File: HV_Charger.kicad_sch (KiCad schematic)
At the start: 25 parts, among them J1 HVIL, J10 G6B-1114P-US-DC24, J11 Banana_Connector, J12 Battery GLV, J2 E-Stop, J3 PP Connector, J4 IMD Indicator, J5 AMS Indicator, J6 CAN, J7 CAN_Expansion1, J8 CAN_Expansion2, J9 DC Input

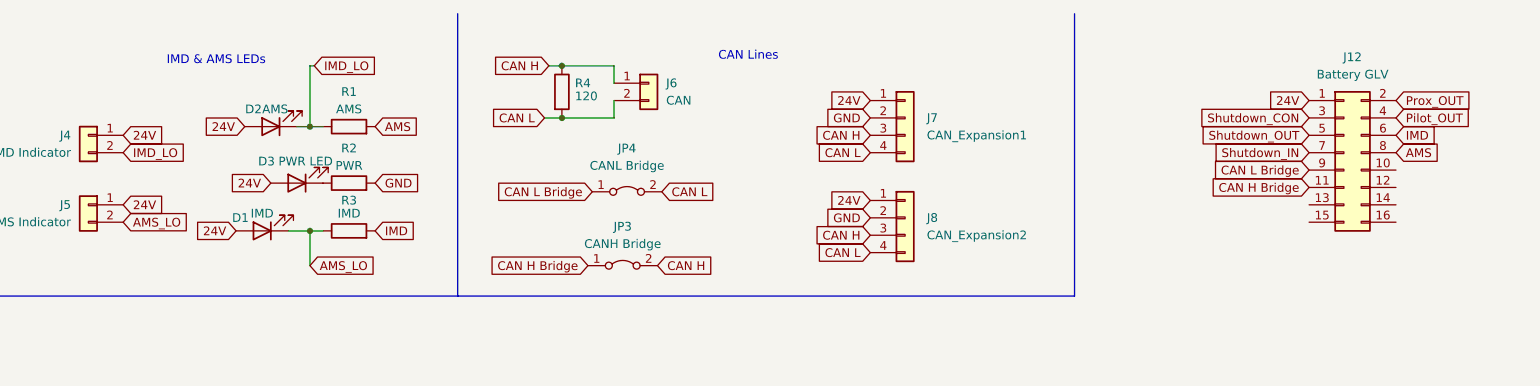
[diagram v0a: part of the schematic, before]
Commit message: more stuff done
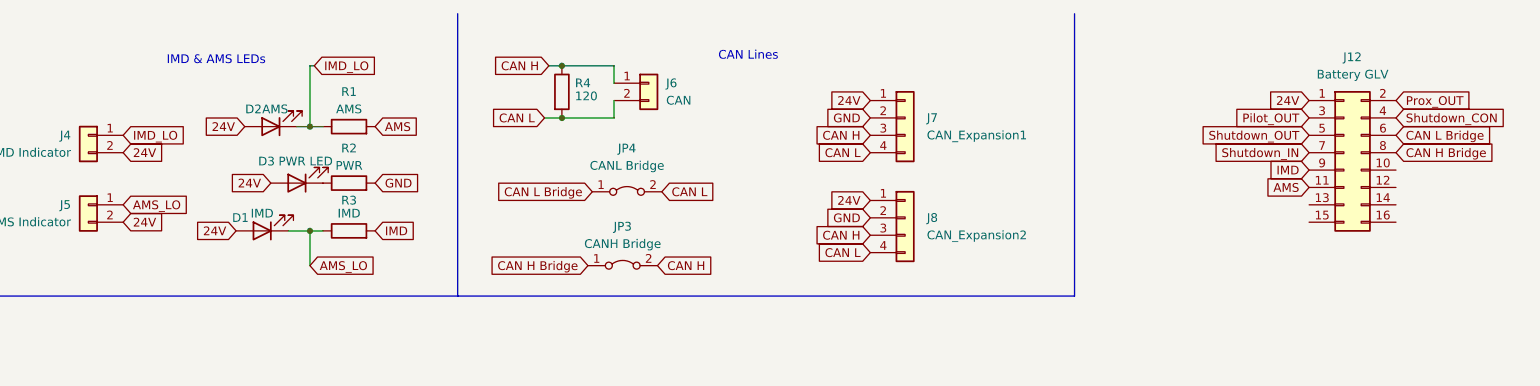
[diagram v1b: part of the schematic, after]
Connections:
- net 24V: now also J4.2 (Pin_2), J5.2 (Pin_2); no longer J4.1 (Pin_1), J5.1 (Pin_1)
- net AMS: now also J12.11 (Pin_11); no longer J12.8 (Pin_8)
- net AMS_LO: now also J5.1 (Pin_1); no longer J5.2 (Pin_2)
- net CAN H Bridge: now also J12.8 (Pin_8); no longer J12.11 (Pin_11)
- net CAN L Bridge: now also J12.6 (Pin_6); no longer J12.9 (Pin_9)
- net IMD: now also J12.9 (Pin_9); no longer J12.6 (Pin_6)
- net IMD_LO: now also J4.1 (Pin_1); no longer J4.2 (Pin_2)
- net Pilot_OUT: now also J12.3 (Pin_3); no longer J12.4 (Pin_4)
- net Shutdown_CON: now also J12.4 (Pin_4); no longer J12.3 (Pin_3)
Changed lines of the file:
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@@
     (effects (font (size 1.27 1.27)) (justify left bottom))
   )
-  (global_label "Pilot_OUT" (shape input) (at 269.24 27.305 0) (fields_autoplaced)
-    (effects (font (size 1.27 1.27)) (justify left))
-    (property "Intersheet References" "${INTERSHEET_REFS}" (id 0) (at 280.6641 27.2256 0)
-      (effects (font (size 1.27 1.27)) (justify left) hide)
-    )
-  )
   (global_label "Shutdown_IN" (shape input) (at 256.54 32.385 180) (fields_autoplaced)
     (effects (font (size 1.27 1.27)) (justify right))
@@
     )
   )
-  (global_label "AMS_LO" (shape input) (at 83.185 42.545 0) (fields_autoplaced)
-    (effects (font (size 1.27 1.27)) (justify left))
-    (property "Intersheet References" "${INTERSHEET_REFS}" (id 0) (at 92.6738 42.4656 0)
-      (effects (font (size 1.27 1.27)) (justify left) hide)
-    )
-  )
   (global_label "GND" (shape input) (at 192.405 41.91 180) (fields_autoplaced)
     (effects (font (size 1.27 1.27)) (justify right))
@@
     )
   )
-  (global_label "CAN H Bridge" (shape input) (at 256.54 37.465 180) (fields_autoplaced)
-    (effects (font (size 1.27 1.27)) (justify right))
-    (property "Intersheet References" "${INTERSHEET_REFS}" (id 0) (at 241.1245 37.3856 0)
-      (effects (font (size 1.27 1.27)) (justify right) hide)
+  (global_label "24V" (shape input) (at 83.185 32.385 0) (fields_autoplaced)
+    (effects (font (size 1.27 1.27)) (justify left))
+    (property "Intersheet References" "${INTERSHEET_REFS}" (id 0) (at 89.1057 32.3056 0)
+      (effects (font (size 1.27 1.27)) (justify left) hide)
     )
   )
@@
     )
   )
+  (global_label "IMD_LO" (shape input) (at 83.185 29.845 0) (fields_autoplaced)
+    (effects (font (size 1.27 1.27)) (justify left))
+    (property "Intersheet References" "${INTERSHEET_REFS}" (id 0) (at 92.2505 29.7656 0)
+      (effects (font (size 1.27 1.27)) (justify left) hide)
+    )
+  )
   (global_label "24V" (shape input) (at 256.54 24.765 180) (fields_autoplaced)
     (effects (font (size 1.27 1.27)) (justify right))
@@
     )
   )
-  (global_label "24V" (shape input) (at 83.185 40.005 0) (fields_autoplaced)
-    (effects (font (size 1.27 1.27)) (justify left))
-    (property "Intersheet References" "${INTERSHEET_REFS}" (id 0) (at 89.1057 39.9256 0)
-      (effects (font (size 1.27 1.27)) (justify left) hide)
-    )
-  )
   (global_label "CAN H" (shape input) (at 192.405 29.845 180) (fields_autoplaced)
     (effects (font (size 1.27 1.27)) (justify right))
@@
     )
   )
+  (global_label "AMS" (shape input) (at 256.54 37.465 180) (fields_autoplaced)
+    (effects (font (size 1.27 1.27)) (justify right))
+    (property "Intersheet References" "${INTERSHEET_REFS}" (id 0) (at 250.3774 37.5444 0)
+      (effects (font (size 1.27 1.27)) (justify right) hide)
+    )
+  )
   (global_label "24V" (shape input) (at 192.405 24.765 180) (fields_autoplaced)
     (effects (font (size 1.27 1.27)) (justify right))
@@
     )
   )
+  (global_label "CAN L Bridge" (shape input) (at 269.24 29.845 0) (fields_autoplaced)
+    (effects (font (size 1.27 1.27)) (justify left))
+    (property "Intersheet References" "${INTERSHEET_REFS}" (id 0) (at 284.3531 29.9244 0)
+      (effects (font (size 1.27 1.27)) (justify left) hide)
+    )
+  )
   (global_label "CAN L Bridge" (shape input) (at 151.765 38.1 180) (fields_autoplaced)
     (effects (font (size 1.27 1.27)) (justify right))
@@
     )
   )
-  (global_label "24V" (shape input) (at 83.185 29.845 0) (fields_autoplaced)
-    (effects (font (size 1.27 1.27)) (justify left))
-    (property "Intersheet References" "${INTERSHEET_REFS}" (id 0) (at 89.1057 29.7656 0)
-      (effects (font (size 1.27 1.27)) (justify left) hide)
-    )
-  )
   (global_label "24V" (shape input) (at 100.965 28.575 180) (fields_autoplaced)
     (effects (font (size 1.27 1.27)) (justify right))
@@
     )
   )
+  (global_label "Shutdown_CON" (shape input) (at 269.24 27.305 0) (fields_autoplaced)
+    (effects (font (size 1.27 1.27)) (justify left))
+    (property "Intersheet References" "${INTERSHEET_REFS}" (id 0) (at 285.5626 27.3844 0)
+      (effects (font (size 1.27 1.27)) (justify left) hide)
+    )
+  )
   (global_label "CAN L" (shape input) (at 192.405 32.385 180) (fields_autoplaced)
     (effects (font (size 1.27 1.27)) (justify right))
@@
     )
   )
+  (global_label "24V" (shape input) (at 83.185 42.545 0) (fields_autoplaced)
+    (effects (font (size 1.27 1.27)) (justify left))
+    (property "Intersheet References" "${INTERSHEET_REFS}" (id 0) (at 89.1057 42.4656 0)
+      (effects (font (size 1.27 1.27)) (justify left) hide)
+    )
+  )
   (global_label "Prox" (shape input) (at 27.94 66.675 180) (fields_autoplaced)
     (effects (font (size 1.27 1.27)) (justify right))
@@
     )
   )
+  (global_label "AMS_LO" (shape input) (at 83.185 40.005 0) (fields_autoplaced)
+    (effects (font (size 1.27 1.27)) (justify left))
+    (property "Intersheet References" "${INTERSHEET_REFS}" (id 0) (at 92.6738 39.9256 0)
+      (effects (font (size 1.27 1.27)) (justify left) hide)
+    )
+  )
   (global_label "Shutdown_OUT" (shape input) (at 256.54 29.845 180) (fields_autoplaced)
     (effects (font (size 1.27 1.27)) (justify right))
@@
     )
   )
+  (global_label "IMD" (shape input) (at 256.54 34.925 180) (fields_autoplaced)
+    (effects (font (size 1.27 1.27)) (justify right))
+    (property "Intersheet References" "${INTERSHEET_REFS}" (id 0) (at 250.8007 35.0044 0)
+      (effects (font (size 1.27 1.27)) (justify right) hide)
+    )
+  )
   (global_label "Prox_OUT" (shape input) (at 269.24 24.765 0) (fields_autoplaced)
     (effects (font (size 1.27 1.27)) (justify left))
@@
     )
   )
-  (global_label "IMD" (shape input) (at 269.24 29.845 0) (fields_autoplaced)
-    (effects (font (size 1.27 1.27)) (justify left))
-    (property "Intersheet References" "${INTERSHEET_REFS}" (id 0) (at 274.9793 29.7656 0)
-      (effects (font (size 1.27 1.27)) (justify left) hide)
-    )
-  )
-  (global_label "Shutdown_CON" (shape input) (at 256.54 27.305 180) (fields_autoplaced)
-    (effects (font (size 1.27 1.27)) (justify right))
-    (property "Intersheet References" "${INTERSHEET_REFS}" (id 0) (at 240.2174 27.2256 0)
+  (global_label "Pilot_OUT" (shape input) (at 256.54 27.305 180) (fields_autoplaced)
+    (effects (font (size 1.27 1.27)) (justify right))
+    (property "Intersheet References" "${INTERSHEET_REFS}" (id 0) (at 245.1159 27.3844 0)
       (effects (font (size 1.27 1.27)) (justify right) hide)
     )
@@
     )
   )
-  (global_label "CAN L Bridge" (shape input) (at 256.54 34.925 180) (fields_autoplaced)
-    (effects (font (size 1.27 1.27)) (justify right))
-    (property "Intersheet References" "${INTERSHEET_REFS}" (id 0) (at 241.4269 34.8456 0)
-      (effects (font (size 1.27 1.27)) (justify right) hide)
-    )
-  )
   (global_label "24V" (shape input) (at 33.655 24.765 0) (fields_autoplaced)
     (effects (font (size 1.27 1.27)) (justify left))
@@
     )
   )
-  (global_label "IMD_LO" (shape input) (at 83.185 32.385 0) (fields_autoplaced)
-    (effects (font (size 1.27 1.27)) (justify left))
-    (property "Intersheet References" "${INTERSHEET_REFS}" (id 0) (at 92.2505 32.3056 0)
-      (effects (font (size 1.27 1.27)) (justify left) hide)
-    )
-  )
   (global_label "Pilot" (shape input) (at 220.345 152.4 180) (fields_autoplaced)
     (effects (font (size 1.27 1.27)) (justify right))
@@
     )
   )
-  (global_label "AMS" (shape input) (at 269.24 32.385 0) (fields_autoplaced)
-    (effects (font (size 1.27 1.27)) (justify left))
-    (property "Intersheet References" "${INTERSHEET_REFS}" (id 0) (at 275.4026 32.3056 0)
-      (effects (font (size 1.27 1.27)) (justify left) hide)
-    )
+  (global_label "CAN H Bridge" (shape input) (at 269.24 32.385 0) (fields_autoplaced)
+    (effects (font (size 1.27 1.27)) (justify left))
+    (property "Intersheet References" "${INTERSHEET_REFS}" (id 0) (at 284.6555 32.4644 0)
+      (effects (font (size 1.27 1.27)) (justify left) hide)
+    )

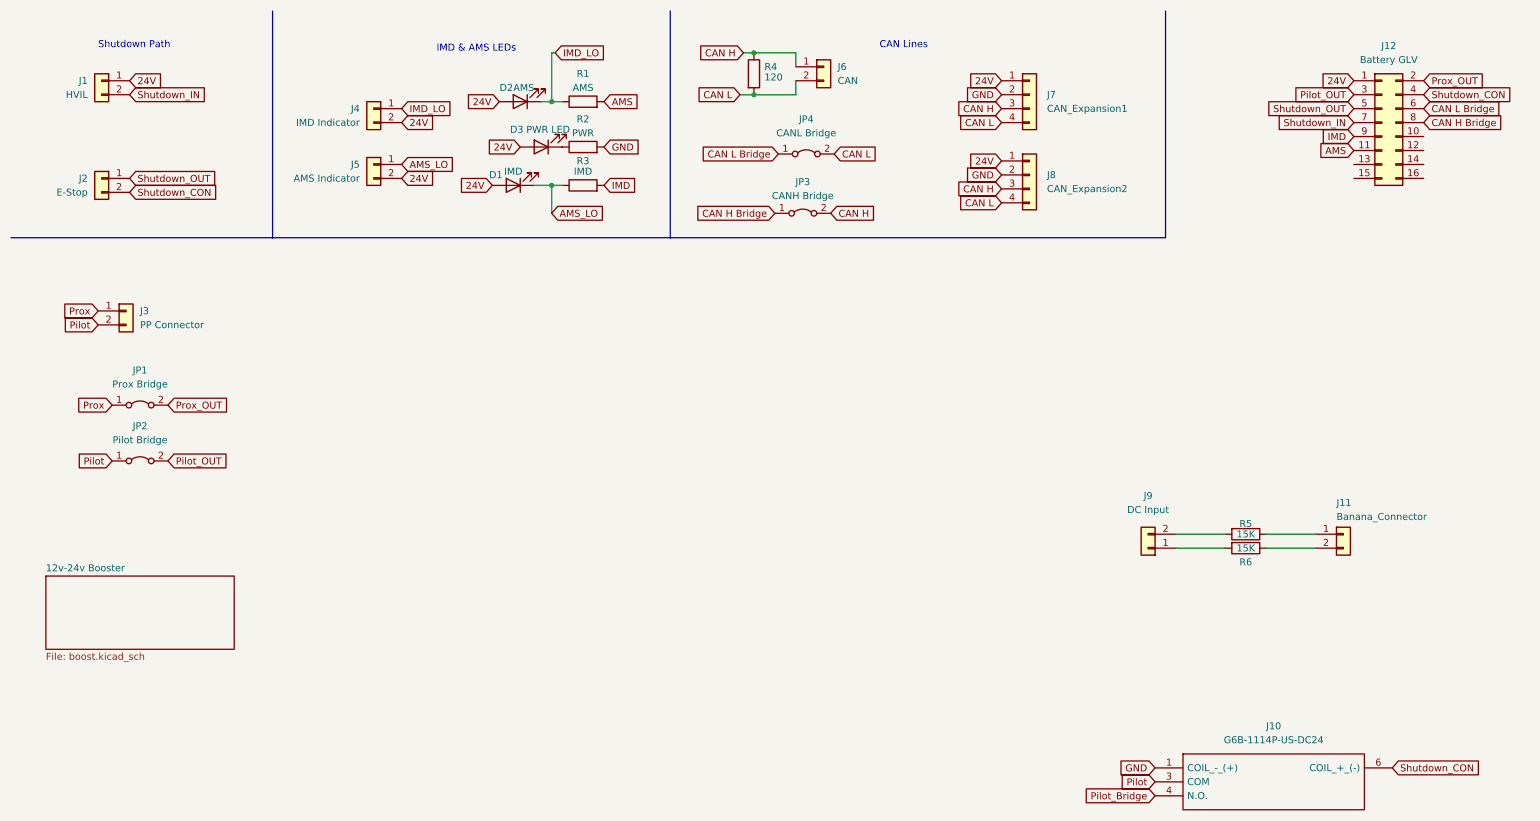
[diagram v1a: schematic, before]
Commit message: Done
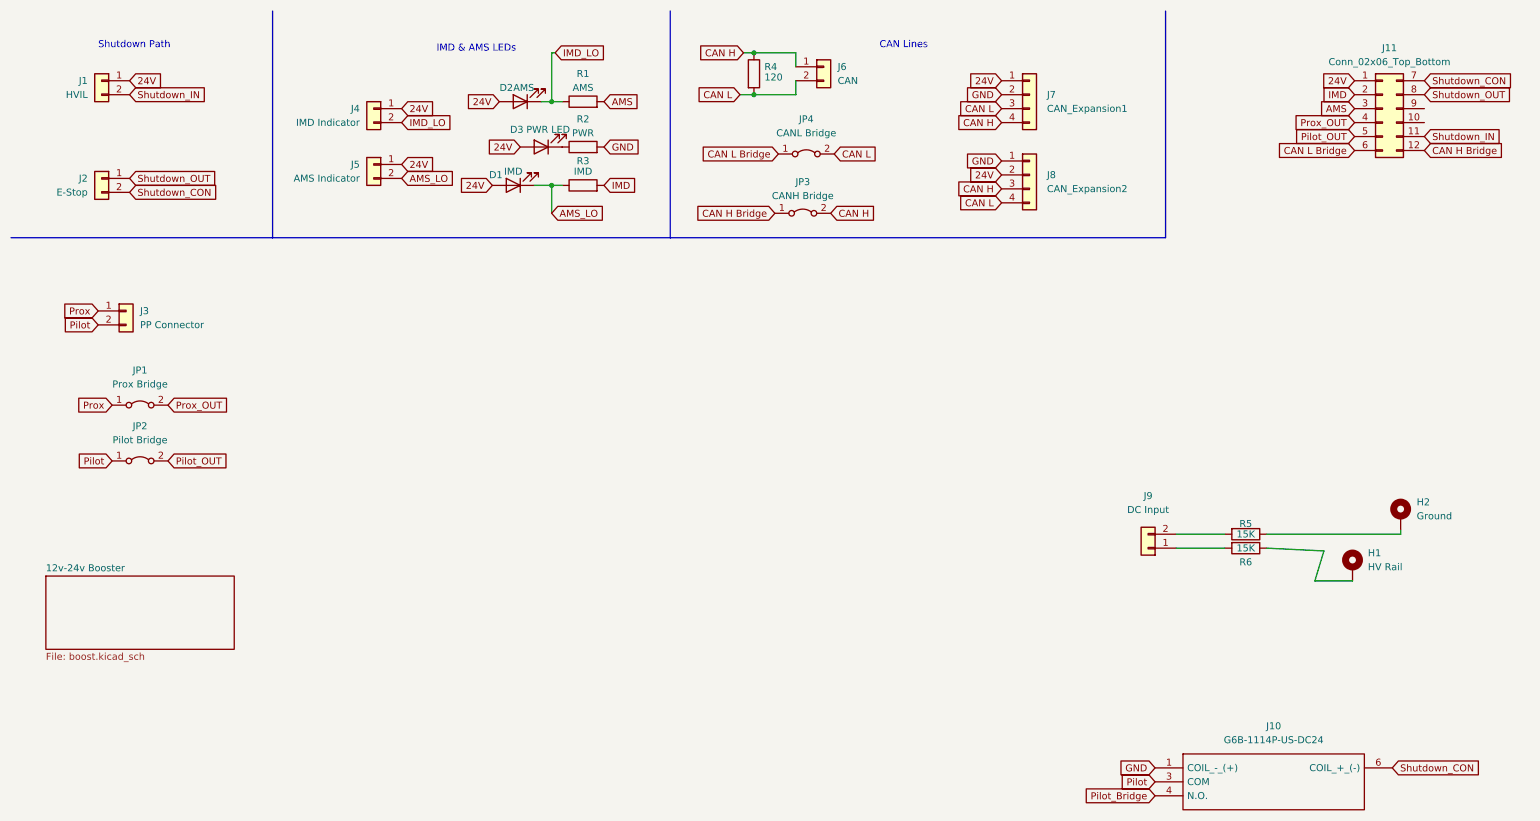
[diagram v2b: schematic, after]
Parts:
- removed J11: Banana_Connector, symbol Connector_Generic:Conn_01x02
- removed J12: Battery GLV, Connector_Molex:Molex_Micro-Fit_3.0_43045-1612_2x08_P3.00mm_Vertical, symbol Connector_Generic:Conn_02x08_Odd_Even
- added H1: HV Rail, Custom:Banana_Jack, symbol Mechanical:MountingHole_Pad
- added H2: Ground, Custom:Banana_Jack, symbol Mechanical:MountingHole_Pad
- added J11: Conn_02x06_Top_Bottom, Connector_Molex:Molex_Micro-Fit_3.0_43045-1212_2x06_P3.00mm_Vertical, symbol Connector_Generic:Conn_02x06_Top_Bottom
- D1, D2, D3: footprint LED_THT:LED_D3.0mm -> LED_SMD:LED_0603_1608Metric
- R1, R2, R3, R4: footprint Resistor_THT:R_Axial_DIN0204_L3.6mm_D1.6mm_P1.90mm_Vertical -> Resistor_SMD:R_0603_1608Metric
- R5, R6: footprint Resistor_THT:R_Axial_DIN0204_L3.6mm_D1.6mm_P1.90mm_Vertical -> SamacSys_Parts:RESC11050X120N
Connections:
- net 24V: now also J4.1 (Pin_1), J5.1 (Pin_1), J8.2 (Pin_2), J11.1 (Pin_1); no longer J4.2 (Pin_2), J5.2 (Pin_2), J8.1 (Pin_1)
- net AMS: now also J11.3 (Pin_3)
- net AMS_LO: now also J5.2 (Pin_2); no longer J5.1 (Pin_1)
- net CAN H: now also J7.4 (Pin_4); no longer J7.3 (Pin_3)
- net CAN H Bridge: now also J11.12 (Pin_12)
- net CAN L: now also J7.3 (Pin_3); no longer J7.4 (Pin_4)
- net CAN L Bridge: now also J11.6 (Pin_6)
- net GND: now also J8.1 (Pin_1); no longer J8.2 (Pin_2)
- net IMD: now also J11.2 (Pin_2)
- net IMD_LO: now also J4.2 (Pin_2); no longer J4.1 (Pin_1)
- net Pilot_OUT: now also J11.5 (Pin_5)
- net Prox_OUT: now also J11.4 (Pin_4)
- net Shutdown_CON: now also J11.7 (Pin_7)
- net Shutdown_IN: now also J11.11 (Pin_11)
- net Shutdown_OUT: now also J11.8 (Pin_8)
- net at R6.1: now also H1.1
- net at R5.1: now also H2.1
